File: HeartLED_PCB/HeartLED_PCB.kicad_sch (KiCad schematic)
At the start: 35 parts, among them U1 ICM7555IBAZ-T, U2 CD4017BM96, U3 TPS61222DCKR, U4 HX SS12F44G4

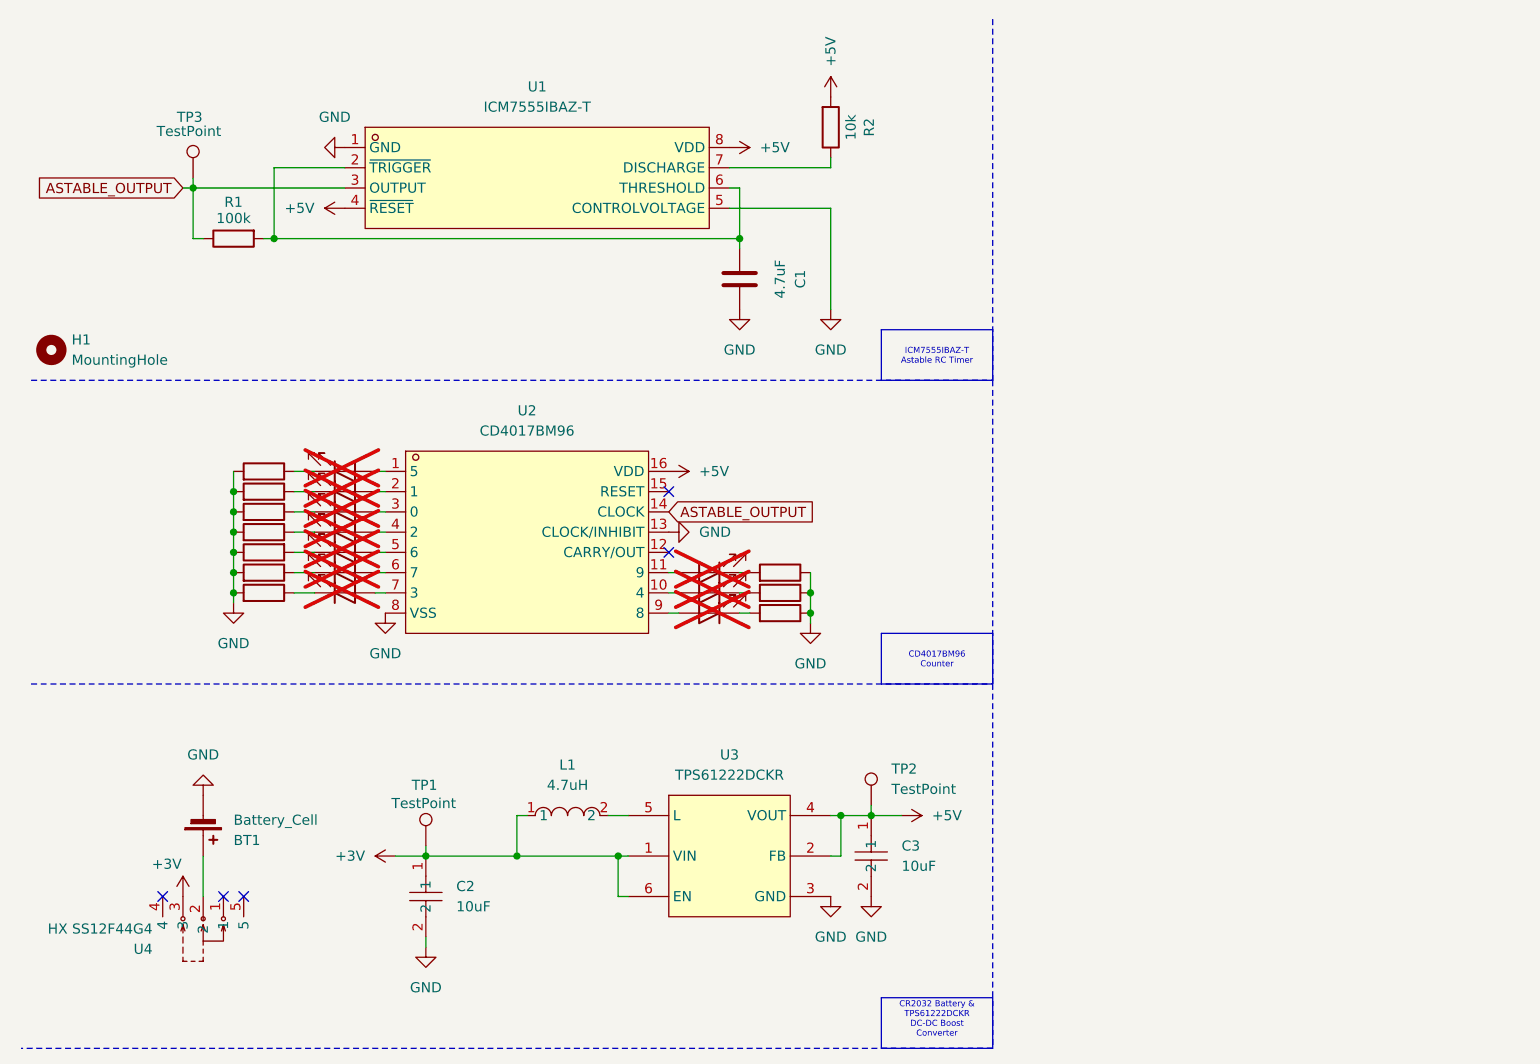
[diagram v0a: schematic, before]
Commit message: Routing done
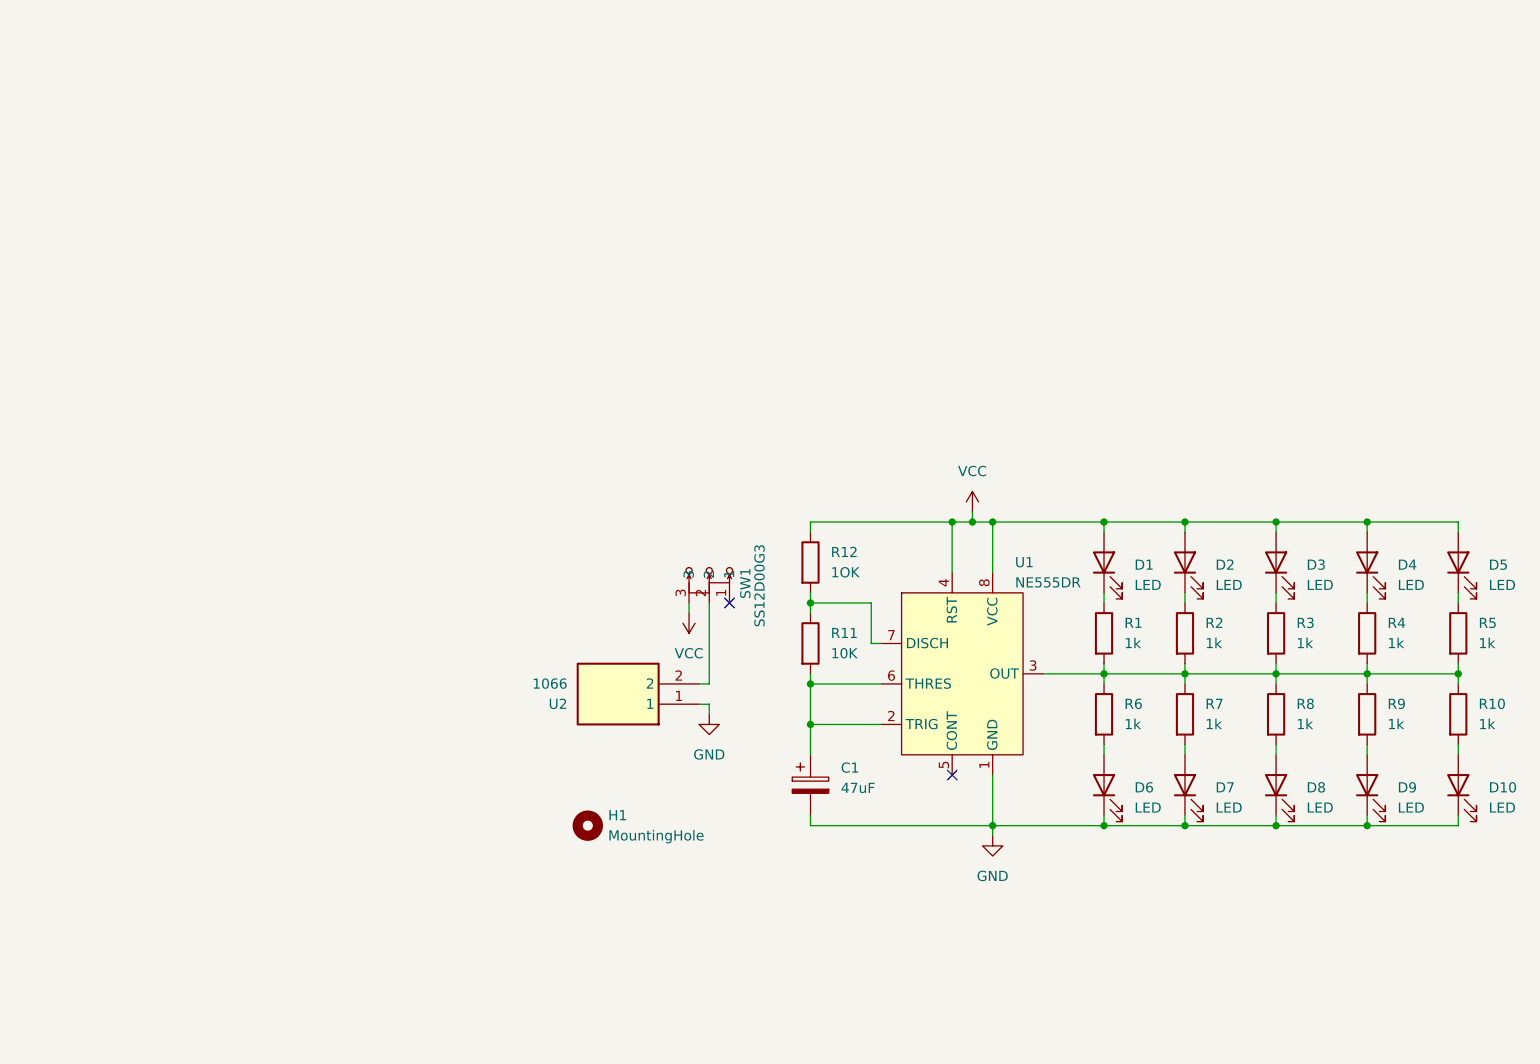
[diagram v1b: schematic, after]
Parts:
- removed BT1: Battery_Cell, Battery:BatteryHolder_Keystone_1060_1x2032, symbol Device:Battery_Cell
- removed C1: 4.7uF, FOOTPRINTS:CL10A475KP8NNNC, symbol Device:C
- removed C2, C3: 10uF, FOOTPRINTS:CL10A106MQ8NNNC, symbol CL10A106MQ8NNNC:CL10A106MQ8NNNC
- removed L1: 4.7uH, FOOTPRINTS:LQH3NPN4R7MMEL, symbol LQH3NPN4R7MMEL:LQH3NPN4R7MMEL
- removed TP1, TP2, TP3: TestPoint, TestPoint:TestPoint_Pad_D1.0mm, symbol Connector:TestPoint
- removed U1: ICM7555IBAZ-T, FOOTPRINTS:ICM7555IBAZ-T, symbol ICM7555IBAZ-T:ICM7555IBAZ-T
- removed U2: CD4017BM96, FOOTPRINTS:CD4017BM96, symbol CD4017BM96:CD4017BM96
- removed U3: TPS61222DCKR, FOOTPRINTS:TPS61222DCKR, symbol TPS61222DCKR:TPS61222DCKR
- removed U4: HX SS12F44G4, FOOTPRINTS:HX SS12F44G4, symbol HXSS12F44G4:HXSS12F44G4
- added C1: 47uF, Capacitor_THT:C_Radial_D5.0mm_H7.0mm_P2.00mm, symbol Device:C_Polarized
- added SW1: SS12D00G3, FOOTPRINTS:SS12D00G3, symbol SS12D00G3:SS12D00G3
- added U1: NE555DR, FOOTPRINTS:NE555DR, symbol NE555DR:NE555DR
- added U2: 1066, FOOTPRINTS:1066, symbol 1066:1066
- D1, D10, D2, D3, D4, D5, D6, D7, D8, D9: now fitted
- H1: footprint MountingHole:MountingHole_2.1mm -> MountingHole:MountingHole_3.2mm_M3
- R1: value 100k -> 1k; footprint FOOTPRINTS:0603WAJ0104T5E -> Resistor_THT:R_Axial_DIN0207_L6.3mm_D2.5mm_P7.62mm_Horizontal; LCSC C15458 -> (none)
- R10, R3, R4, R5, R6, R7, R8, R9: value 3.3k -> 1k; footprint FOOTPRINTS:0402WGJ0332TCE -> Resistor_THT:R_Axial_DIN0207_L6.3mm_D2.5mm_P7.62mm_Horizontal; LCSC C25936 -> (none)
- R11: value 3.3k -> 10K; footprint FOOTPRINTS:0402WGJ0332TCE -> Resistor_THT:R_Axial_DIN0207_L6.3mm_D2.5mm_P7.62mm_Horizontal; LCSC C25936 -> (none)
- R12: value 3.3k -> 1OK; footprint FOOTPRINTS:0402WGJ0332TCE -> Resistor_THT:R_Axial_DIN0207_L6.3mm_D2.5mm_P7.62mm_Horizontal; LCSC C25936 -> (none)
- R2: value 10k -> 1k; footprint FOOTPRINTS:0402WGJ0103TCE -> Resistor_THT:R_Axial_DIN0207_L6.3mm_D2.5mm_P7.62mm_Horizontal; LCSC C25531 -> (none)
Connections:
- net +5V is gone; now on an unnamed net: R2.2
- net ASTABLE_OUTPUT is gone; now on an unnamed net: R1.1
- net GND: now also D10.1 (K), D6.1 (K), D7.1 (K), D8.1 (K), D9.1 (K), C1.2, U1.1 (GND), U2.1; no longer R10.1, R11.1, R12.1, R3.2, R4.2, R5.2, R6.2, R7.1, R8.2, R9.2
- net VCC: now reaches D1.2 (A)
- net VCC: now also D2.2 (A), D3.2 (A), D4.2 (A), D5.2 (A), R12.1, SW1.3, U1.4 (RST), U1.8 (VCC)
- net at D9.2 (A): now also R9.2
- net at D10.2 (A): now also R10.2
- net at D6.2 (A): now also R6.2
- net at D7.2 (A): now also R7.2
- net at D8.2 (A): now also R8.2
- net at R8.1: now also R1.2, R10.1, R3.2, R4.2, R5.2, R6.1, R7.1, R9.1, U1.3 (OUT); no longer D6.1 (K)
- net at D1.1 (K): no longer R3.1
- net at D3.1 (K): now also R3.1; no longer R5.1
- net at R12.2: now also R11.1, U1.7 (DISCH); no longer D10.1 (K)
- net at R11.2: now also C1.1, U1.2 (TRIG), U1.6 (THRES); no longer D9.1 (K)
- net at D5.1 (K): now also R5.1; no longer R7.2
- net at R4.1: now also D4.1 (K); no longer D2.1 (K)
- net at R2.1: now also D2.1 (K)
- new net: SW1.2, U2.2
- no-connect marks 5 -> 2
